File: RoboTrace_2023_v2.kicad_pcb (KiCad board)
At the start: 2 copper layers, 110 x 61.2 mm, 165 parts, among them J1 Battery, J10 MOTOR, J11 LINE_SENS, J12 EMCODER_2, J13 SIDE_SENSE_1, J14 SIDE_SENSE_2, J15 SIDE_SENSE_1, J16 FAN_1, J17 SIDE_SENSE_2, J18 FAN_1, J19 POTENTIOMETER, J2 SWD, J3 USART, J4 I2C, J5 STEER_MOTOR, J6 LINE_SENS, J7 EMCODER_1, J8 1S, J9 MOTOR, Q1 PMOS, Q2 TRMT, Q3 TRMT, Q4 TRMT, Q5 TRMT, Q6 A03400A, Q7 TRMT, Q8 TRMT, Q9 A03400A, SW1 RST_SW, SW2 SW_POWER, SW3 SW_1, SW4 SW_2, SW5 SW_3, U1 ICM20649, U10 S7136, U2 STM32F405RGTx, U3 LXDC55F, U4 DSC6021CI2A, U5 DRV8876, U6 NJU7223, U7 DRV8874, U8 DRV8874, U9 S7136

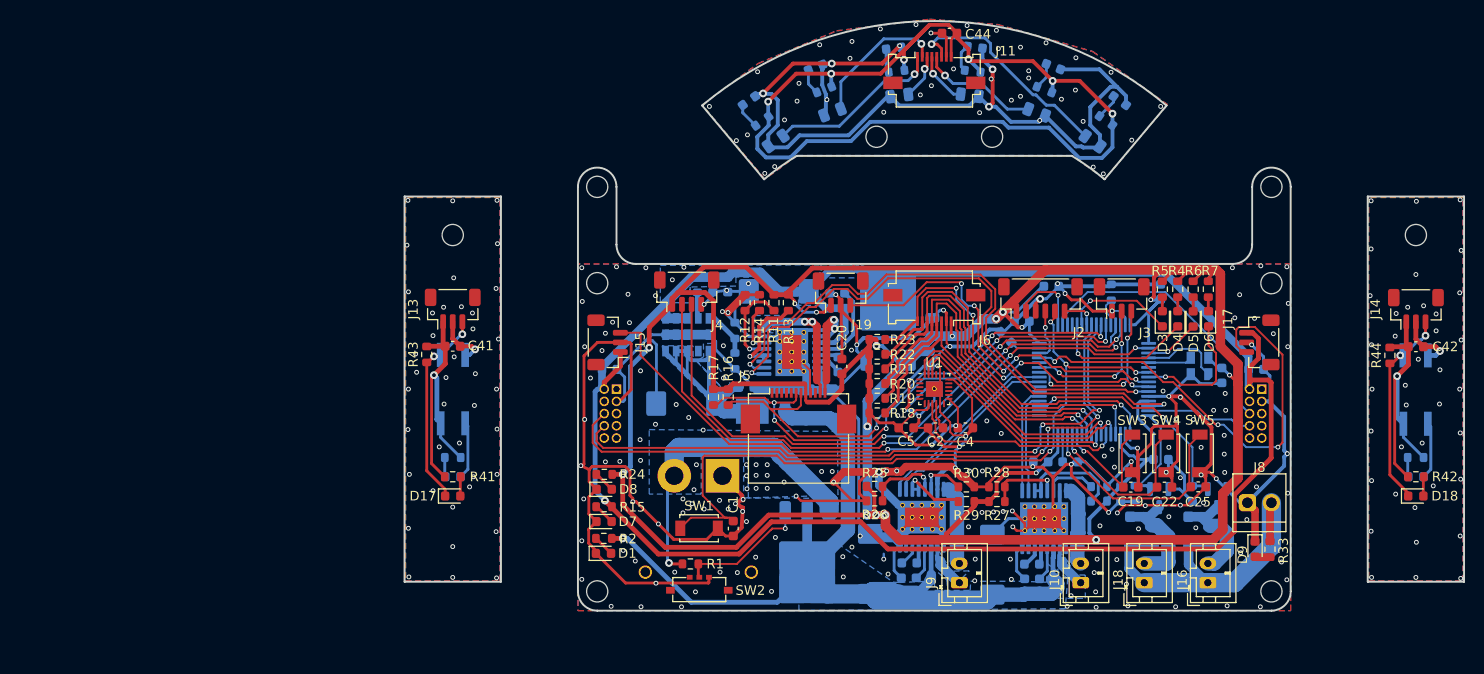
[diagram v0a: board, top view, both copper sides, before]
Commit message: third commit
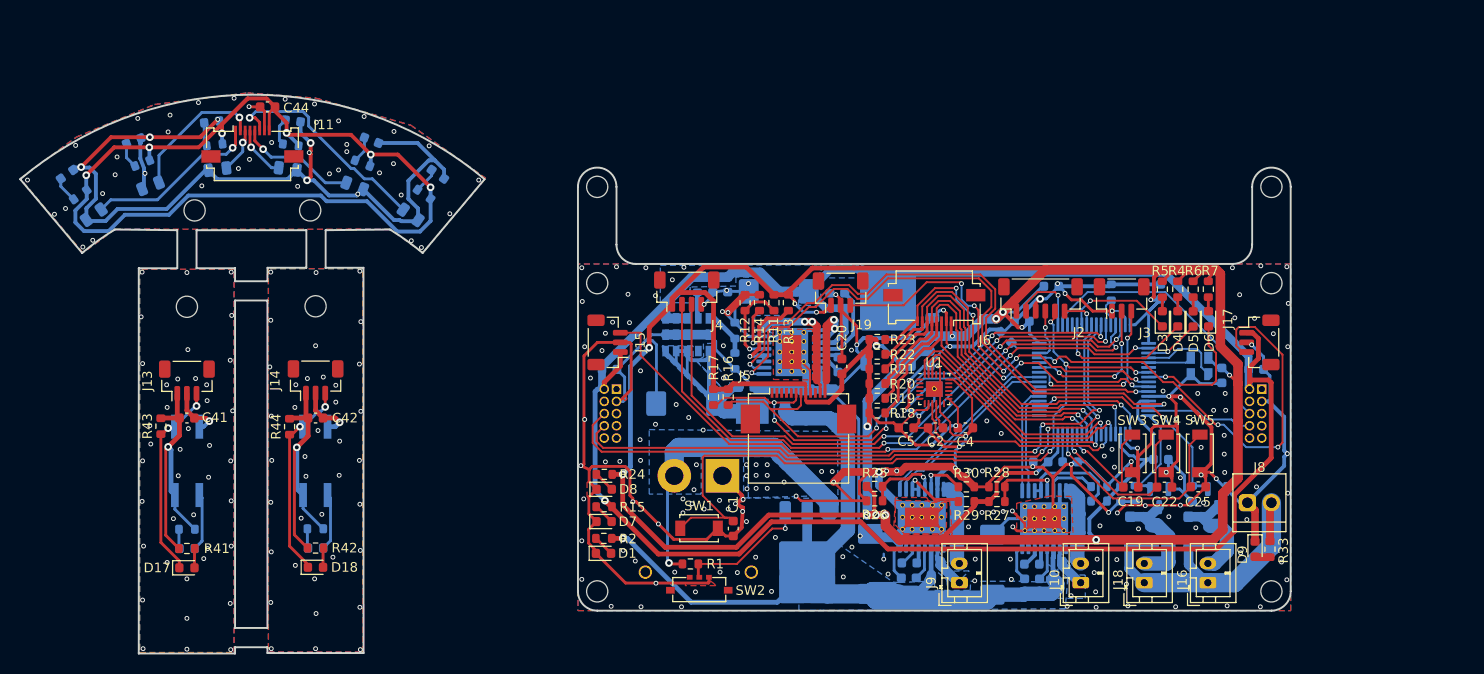
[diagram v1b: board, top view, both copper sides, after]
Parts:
- moved D18 114.5 mm to (85.7, 118.5)
- moved R44 114.5 mm to (83.1, 103.9)
- moved C42 114.5 mm to (85.8, 103.0)
- moved D14 114.5 mm to (85.8, 116.5)
- moved J14 114.5 mm to (85.8, 99.1)
- moved R38 114.5 mm to (85.7, 114.5)
- moved R42 114.5 mm to (85.8, 116.5)
- moved REF** 114.5 mm to (85.8, 91.4)
- moved U10 114.5 mm to (85.7, 107.5)
- moved R36 71.2 mm to (75.3, 74.6)
- moved R45 71.2 mm to (90.6, 76.6)
- moved D10 71.2 mm to (60.0, 77.7)
- moved D11 71.2 mm to (66.9, 74.2)
- moved D12 71.2 mm to (75.0, 72.3)
- moved D21 71.2 mm to (98.5, 77.7)
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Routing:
- net ADC3: track 37.4 -> 36.8 mm
- net ADC6: track 39.5 -> 39.0 mm
- net ADC5: track 40.2 -> 39.7 mm
- net ADC4: track 39.7 -> 39.2 mm
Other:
- board size 110 x 61.2 mm -> 131.9 x 58 mm
